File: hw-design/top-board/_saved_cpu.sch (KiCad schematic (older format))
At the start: 28 parts, among them P4 BOTTOM_CONN, Q1 2N7002, SW1 BT_RESET, U3 MCP6001, U4 LPC1759FBD80, Y1 10MHz

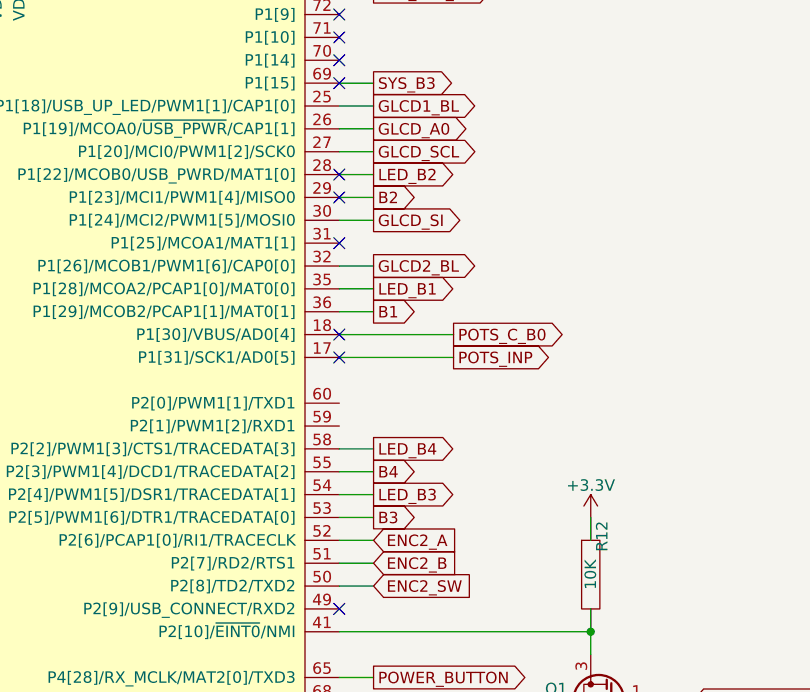
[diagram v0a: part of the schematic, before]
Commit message: sketch route of the components
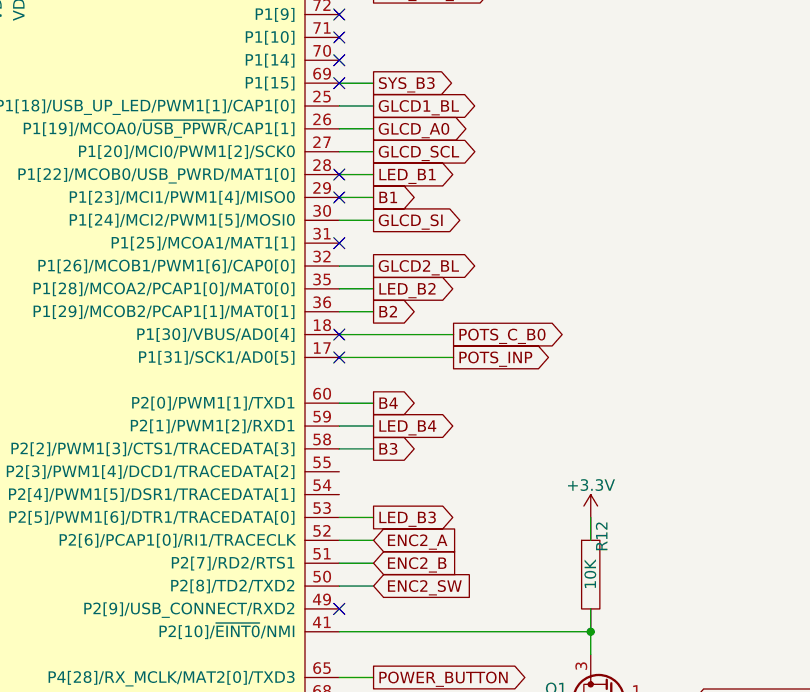
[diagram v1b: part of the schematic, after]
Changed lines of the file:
@@
 Text GLabel 9000 2150 2    50   Output ~ 0
 LED_SYS_B1
+Text GLabel 9000 3650 2    50   Output ~ 0
+LED_B2
+Text GLabel 9000 3250 2    50   Output ~ 0
+B1
+Text GLabel 9000 3750 2    50   Output ~ 0
+B2
 Text GLabel 9000 3150 2    50   Output ~ 0
-LED_B2
-Text GLabel 9000 3750 2    50   Output ~ 0
-B1
-Text GLabel 9000 3250 2    50   Output ~ 0
-B2
-Text GLabel 9000 3650 2    50   Output ~ 0
 LED_B1
 Wire Wire Line
@@
 	9350 3850 8850 3850
 Wire Wire Line
-	9000 3250 8850 3250
-Wire Wire Line
-	9000 3650 8850 3650
-Wire Wire Line
 	9000 2350 8850 2350
-Text GLabel 9000 4450 2    50   Output ~ 0
+Text GLabel 9000 4150 2    50   Output ~ 0
 B4
+Text GLabel 9000 4350 2    50   Output ~ 0
+B3
 Text GLabel 9000 4650 2    50   Output ~ 0
-B3
-Text GLabel 9000 4550 2    50   Output ~ 0
 LED_B3
-Text GLabel 9000 4350 2    50   Output ~ 0
+Text GLabel 9000 4250 2    50   Output ~ 0
 LED_B4
-Wire Wire Line
-	9000 3150 8850 3150
-Wire Wire Line
-	9000 3750 8850 3750
 Connection ~ 2200 1300
 Connection ~ 2200 1200
@@
 	3600 2150 3600 2300
 Wire Wire Line
-	9000 4650 8850 4650
-Wire Wire Line
-	9000 4550 8850 4550
-Wire Wire Line
-	9000 4450 8850 4450
-Wire Wire Line
-	9000 4350 8850 4350
-Wire Wire Line
 	6500 800  6500 950
 Wire Wire Line
@@
 Wire Wire Line
 	9000 2750 8850 2750
+Wire Wire Line
+	9000 4150 8850 4150
+Wire Wire Line
+	9000 4250 8850 4250
+Wire Wire Line
+	9000 4350 8850 4350
+Wire Wire Line
+	9000 4650 8850 4650
+Wire Wire Line
+	9000 3150 8850 3150
+Wire Wire Line
+	9000 3250 8850 3250
+Wire Wire Line
+	9000 3650 8850 3650
+Wire Wire Line
+	9000 3750 8850 3750
 $EndSCHEMATC
